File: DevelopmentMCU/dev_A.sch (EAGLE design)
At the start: 3 parts, among them U1 TM4C123_DEVICE, U2 AP2112K-3.3TRG1

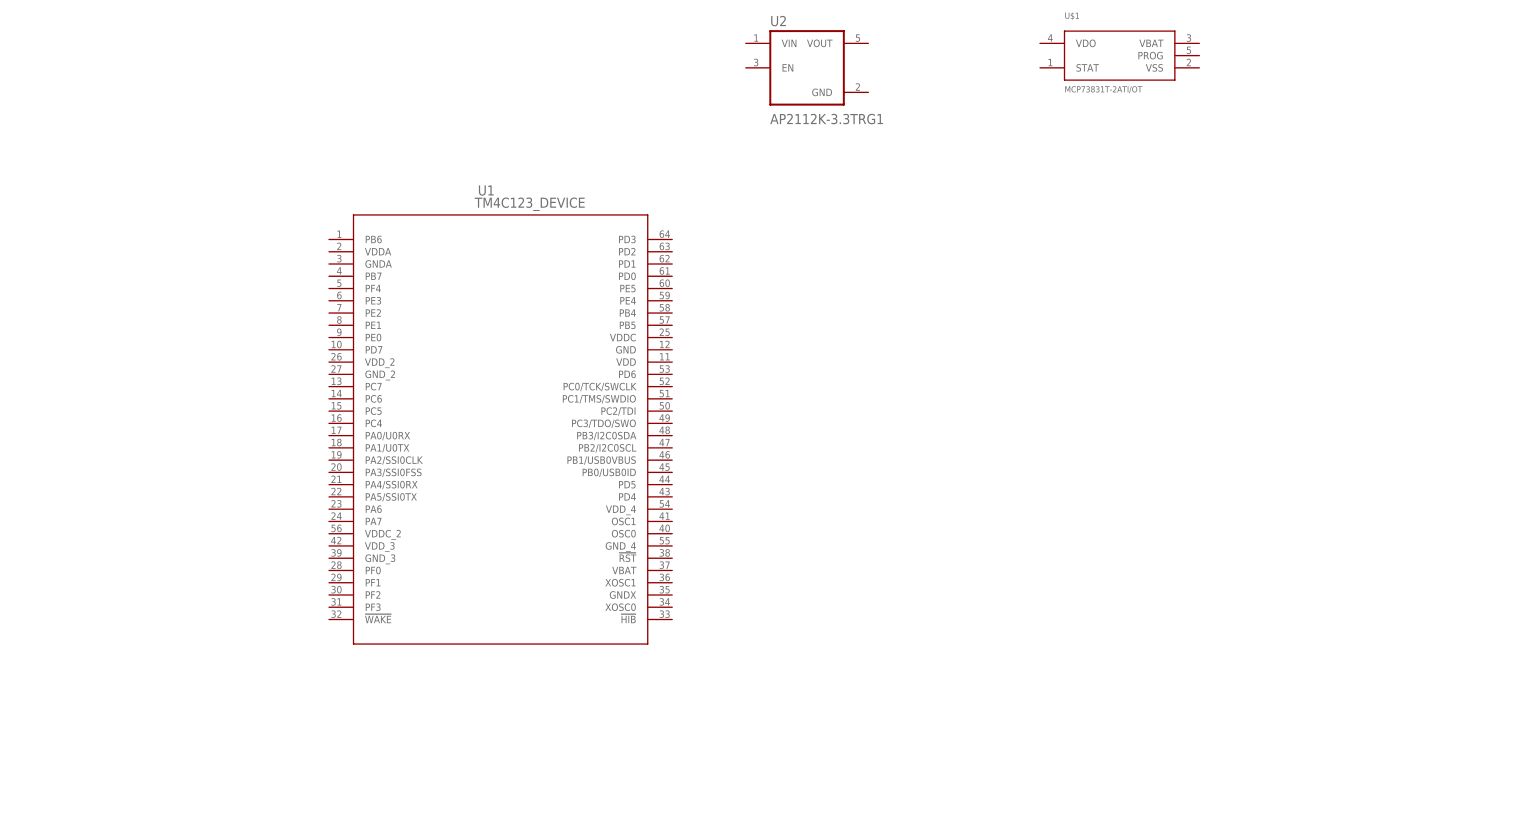
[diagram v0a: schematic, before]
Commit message: Library almost finished
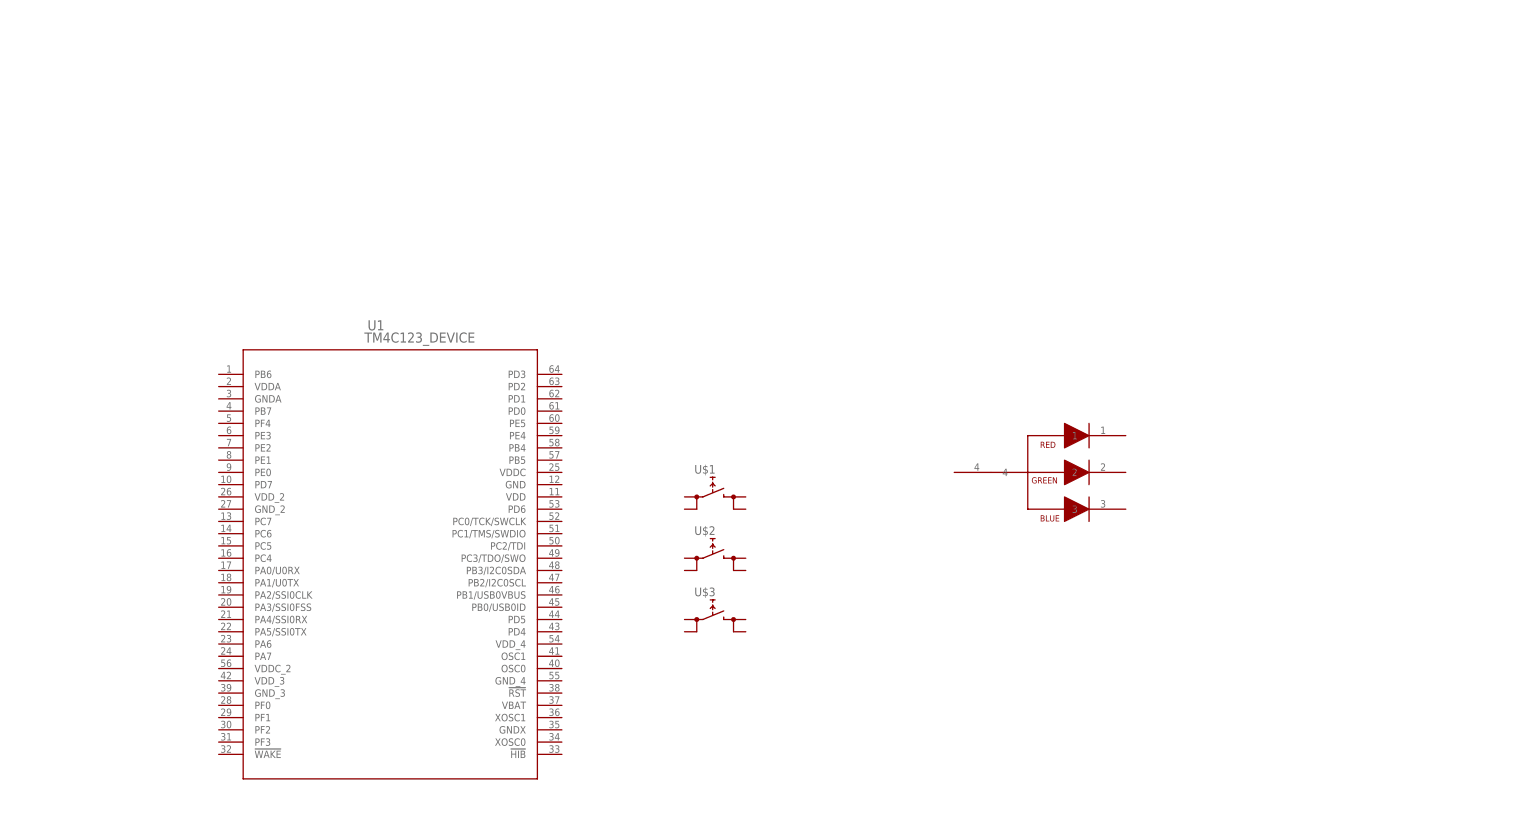
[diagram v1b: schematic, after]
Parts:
- removed U2: AP2112K-3.3TRG1, AP2112K-3.3TRG1:AP2112K-3.3TRG1
- added U$2, U$3: (no value), MICROCONTROLLER:SWITCH_B3S
- added U$4: (no value), MICROCONTROLLER:RGBLED
- U$1: value MCP73831T-2ATI/OT -> (none); device MICROCONTROLLER:MCP73831T-2ATI/OT -> MICROCONTROLLER:SWITCH_B3S
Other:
- moved on the sheet: U1
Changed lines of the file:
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@@
 <layers>
 <layer number="1" name="Top" color="4" fill="1" visible="no" active="no"/>
-<layer number="2" name="Route2" color="16" fill="1" visible="no" active="no"/>
-<layer number="3" name="Route3" color="17" fill="1" visible="no" active="no"/>
-<layer number="4" name="Route4" color="18" fill="1" visible="no" active="no"/>
-<layer number="5" name="Route5" color="19" fill="1" visible="no" active="no"/>
-<layer number="6" name="Route6" color="25" fill="1" visible="no" active="no"/>
-<layer number="7" name="Route7" color="26" fill="1" visible="no" active="no"/>
-<layer number="8" name="Route8" color="27" fill="1" visible="no" active="no"/>
-<layer number="9" name="Route9" color="28" fill="1" visible="no" active="no"/>
-<layer number="10" name="Route10" color="29" fill="1" visible="no" active="no"/>
-<layer number="11" name="Route11" color="30" fill="1" visible="no" active="no"/>
-<layer number="12" name="Route12" color="20" fill="1" visible="no" active="no"/>
-<layer number="13" name="Route13" color="21" fill="1" visible="no" active="no"/>
-<layer number="14" name="Route14" color="22" fill="1" visible="no" active="no"/>
-<layer number="15" name="Route15" color="23" fill="1" visible="no" active="no"/>
+<layer number="2" name="Route2" color="1" fill="3" visible="no" active="no"/>
+<layer number="3" name="Route3" color="4" fill="3" visible="no" active="no"/>
+<layer number="4" name="Route4" color="1" fill="4" visible="no" active="no"/>
+<layer number="5" name="Route5" color="4" fill="4" visible="no" active="no"/>
+<layer number="6" name="Route6" color="1" fill="8" visible="no" active="no"/>
+<layer number="7" name="Route7" color="4" fill="8" visible="no" active="no"/>
+<layer number="8" name="Route8" color="1" fill="2" visible="no" active="no"/>
+<layer number="9" name="Route9" color="4" fill="2" visible="no" active="no"/>
+<layer number="10" name="Route10" color="1" fill="7" visible="no" active="no"/>
+<layer number="11" name="Route11" color="4" fill="7" visible="no" active="no"/>
+<layer number="12" name="Route12" color="1" fill="5" visible="no" active="no"/>
+<layer number="13" name="Route13" color="4" fill="5" visible="no" active="no"/>
+<layer number="14" name="Route14" color="1" fill="6" visible="no" active="no"/>
+<layer number="15" name="Route15" color="4" fill="6" visible="no" active="no"/>
 <layer number="16" name="Bottom" color="1" fill="1" visible="no" active="no"/>
 <layer number="17" name="Pads" color="2" fill="1" visible="no" active="no"/>
 <layer number="18" name="Vias" color="2" fill="1" visible="no" active="no"/>
 <layer number="19" name="Unrouted" color="6" fill="1" visible="no" active="no"/>
-<layer number="20" name="Dimension" color="24" fill="1" visible="no" active="no"/>
+<layer number="20" name="Dimension" color="15" fill="1" visible="no" active="no"/>
 <layer number="21" name="tPlace" color="7" fill="1" visible="no" active="no"/>
 <layer number="22" name="bPlace" color="7" fill="1" visible="no" active="no"/>
@@
 <layer number="97" name="Info" color="7" fill="1" visible="yes" active="yes"/>
 <layer number="98" name="Guide" color="6" fill="1" visible="yes" active="yes"/>
+<layer number="99" name="SpiceOrder" color="7" fill="1" visible="yes" active="yes"/>
 </layers>
 <schematic xreflabel="%F%N/%S.%C%R" xrefpart="/%S.%C%R">
@@
 </classes>
 <parts>
+<part name="FRAME1" library="frames" library_urn="urn:adsk.eagle:library:229" deviceset="FRAME_B_L" device=""/>
 <part name="U1" library="MICROCONTROLLER" deviceset="TM4C123_DEVICE" device="" package3d_urn="urn:adsk.eagle:package:14363313/1"/>
-<part name="FRAME1" library="frames" library_urn="urn:adsk.eagle:library:229" deviceset="FRAME_B_L" device=""/>
-<part name="U2" library="AP2112K-3.3TRG1" deviceset="AP2112K-3.3TRG1" device=""/>
-<part name="U$1" library="MICROCONTROLLER" deviceset="MCP73831T-2ATI/OT" device="" package3d_urn="urn:adsk.eagle:package:14364640/1"/>
+<part name="U$1" library="MICROCONTROLLER" deviceset="SWITCH_B3S" device=""/>
+<part name="U$2" library="MICROCONTROLLER" deviceset="SWITCH_B3S" device=""/>
+<part name="U$3" library="MICROCONTROLLER" deviceset="SWITCH_B3S" device=""/>
+<part name="U$4" library="MICROCONTROLLER" deviceset="RGBLED" device=""/>
 </parts>
 <sheets>
@@
 </plain>
 <instances>
-<instance part="U1" gate="A" x="96.52" y="195.58" smashed="yes">
-<attribute name="NAME" x="129.8956" y="204.6986" size="2.0828" layer="95" ratio="6" rot="SR0"/>
-<attribute name="VALUE" x="129.2606" y="202.1586" size="2.0828" layer="96" ratio="6" rot="SR0"/>
-</instance>
 <instance part="FRAME1" gate="G$1" x="0" y="0" smashed="yes"/>
 <instance part="FRAME1" gate="G$2" x="325.12" y="0" smashed="yes">
@@
 <attribute name="DRAWING_NAME" x="342.9" y="19.05" size="2.54" layer="94"/>
 </instance>
-<instance part="U2" gate="G$1" x="198.12" y="231.14" smashed="yes">
-<attribute name="NAME" x="190.45705" y="239.787609375" size="2.08946875" layer="95" ratio="10" rot="SR0"/>
-<attribute name="VALUE" x="190.4711" y="219.4893" size="2.0883" layer="96" ratio="10" rot="SR0"/>
+<instance part="U1" gate="A" x="73.66" y="167.64" smashed="yes">
+<attribute name="NAME" x="107.0356" y="176.7586" size="2.0828" layer="95" ratio="6" rot="SR0"/>
+<attribute name="VALUE" x="106.4006" y="174.2186" size="2.0828" layer="96" ratio="6" rot="SR0"/>
 </instance>
-<instance part="U$1" gate="A" x="259.08" y="220.98" smashed="yes">
-<attribute name="NAME" x="251.46" y="241.3" size="1.27" layer="95"/>
-<attribute name="VALUE" x="251.46" y="226.06" size="1.27" layer="96"/>
+<instance part="U$1" gate="A" x="177.8" y="142.24" smashed="yes">
+<attribute name="NAME" x="174.752" y="147.066" size="1.778" layer="95"/>
+<attribute name="VALUE" x="173.99" y="136.652" size="1.778" layer="96"/>
 </instance>
+<instance part="U$2" gate="A" x="177.8" y="129.54" smashed="yes">
+<attribute name="NAME" x="174.752" y="134.366" size="1.778" layer="95"/>
+<attribute name="VALUE" x="173.99" y="123.952" size="1.778" layer="96"/>
+</instance>
+<instance part="U$3" gate="A" x="177.8" y="116.84" smashed="yes">
+<attribute name="NAME" x="174.752" y="121.666" size="1.778" layer="95"/>
+<attribute name="VALUE" x="173.99" y="111.252" size="1.778" layer="96"/>
+</instance>
+<instance part="U$4" gate="A" x="271.78" y="144.78" smashed="yes"/>
 </instances>
 <busses>

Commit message: second commit
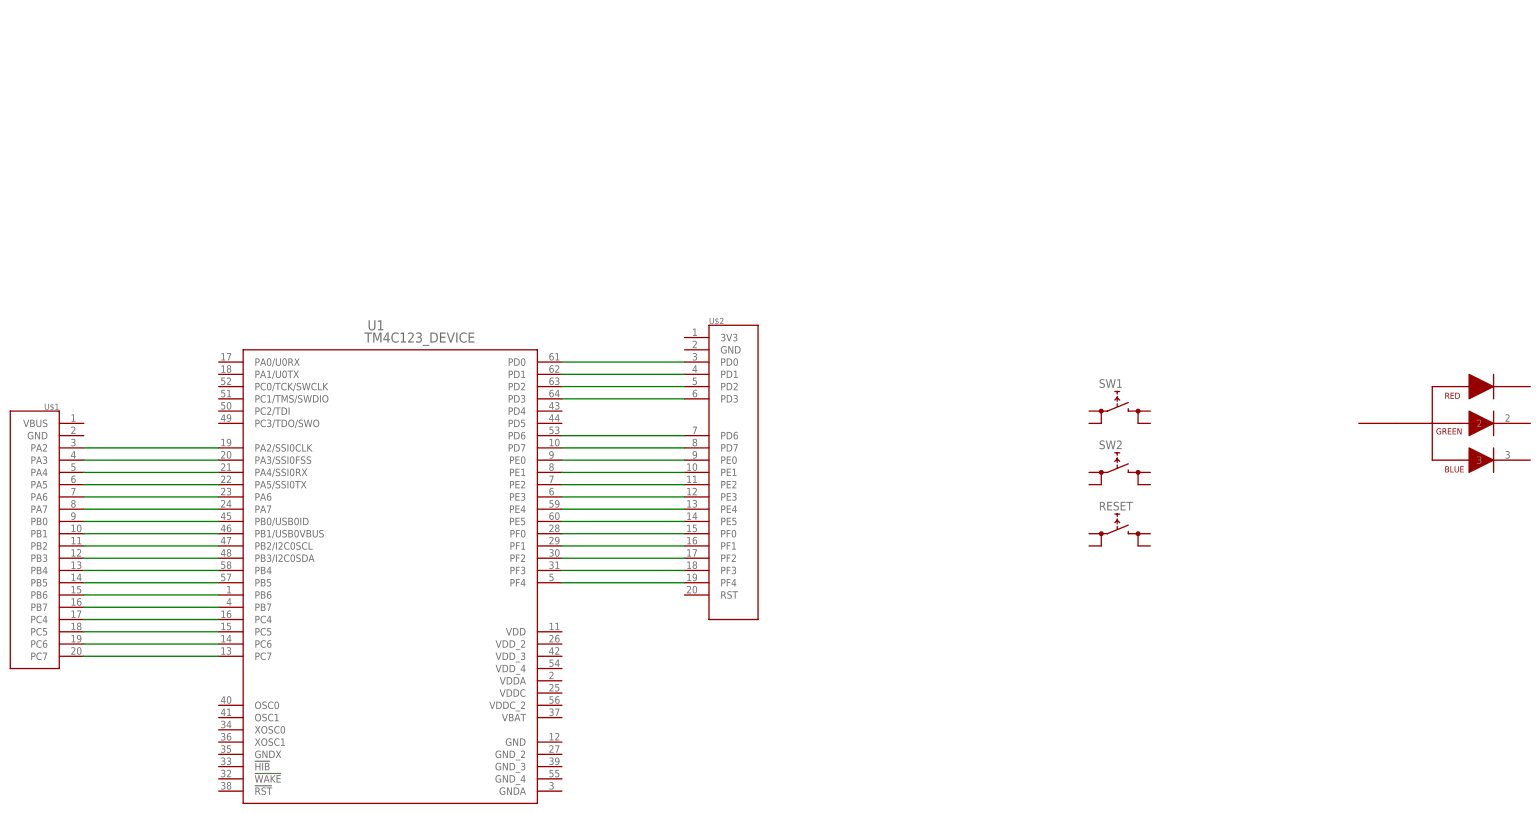
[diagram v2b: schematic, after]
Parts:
- removed U$3: (no value), MICROCONTROLLER:SWITCH_B3S
- added RESET, SW1, SW2: (no value), MICROCONTROLLER:SWITCH_B3S
- U$1: device MICROCONTROLLER:SWITCH_B3S -> MICROCONTROLLER:HEADER_J1
- U$2: device MICROCONTROLLER:SWITCH_B3S -> MICROCONTROLLER:HEADER_J2
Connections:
- new net N$1: U$1.PA2, U1.PA2/SSI0CLK
- new net N$10: U$1.PB3, U1.PB3/I2C0SDA
- new net N$11: U$1.PB4, U1.PB4
- new net N$12: U$1.PB5, U1.PB5
- new net N$13: U$1.PB6, U1.PB6
- new net N$14: U$1.PB7, U1.PB7
- new net N$15: U$1.PC4, U1.PC4
- new net N$16: U$1.PC5, U1.PC5
- new net N$17: U$1.PC6, U1.PC6
- new net N$18: U$1.PC7, U1.PC7
- new net N$19: U$2.PD0, U1.PD0
- new net N$2: U$1.PA3, U1.PA3/SSI0FSS
- new net N$20: U$2.PD1, U1.PD1
- new net N$21: U$2.PD2, U1.PD2
- new net N$22: U$2.PD3, U1.PD3
- new net N$23: U$2.PD6, U1.PD6
- new net N$24: U$2.PD7, U1.PD7
- new net N$25: U$2.PE0, U1.PE0
- new net N$26: U$2.PE1, U1.PE1
- new net N$27: U$2.PE2, U1.PE2
- new net N$28: U$2.PE3, U1.PE3
- new net N$29: U$2.PE4, U1.PE4
- new net N$3: U$1.PA4, U1.PA4/SSI0RX
- new net N$30: U$2.PE5, U1.PE5
- new net N$31: U$2.PF0, U1.PF0
- new net N$32: U$2.PF1, U1.PF1
- new net N$33: U$2.PF2, U1.PF2
- new net N$34: U$2.PF3, U1.PF3
- new net N$35: U$2.PF4, U1.PF4
- new net N$4: U$1.PA5, U1.PA5/SSI0TX
- new net N$5: U$1.PA6, U1.PA6
- new net N$6: U$1.PA7, U1.PA7
- new net N$7: U$1.PB0, U1.PB0/USB0ID
- new net N$8: U$1.PB1, U1.PB1/USB0VBUS
- new net N$9: U$1.PB2, U1.PB2/I2C0SCL
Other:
- moved on the sheet: U1
